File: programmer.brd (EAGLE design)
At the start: 41.1 x 23 mm, 20 parts, among them IC1 74ABT125DB, U1 ATMEGA8U2, X1 16MHz

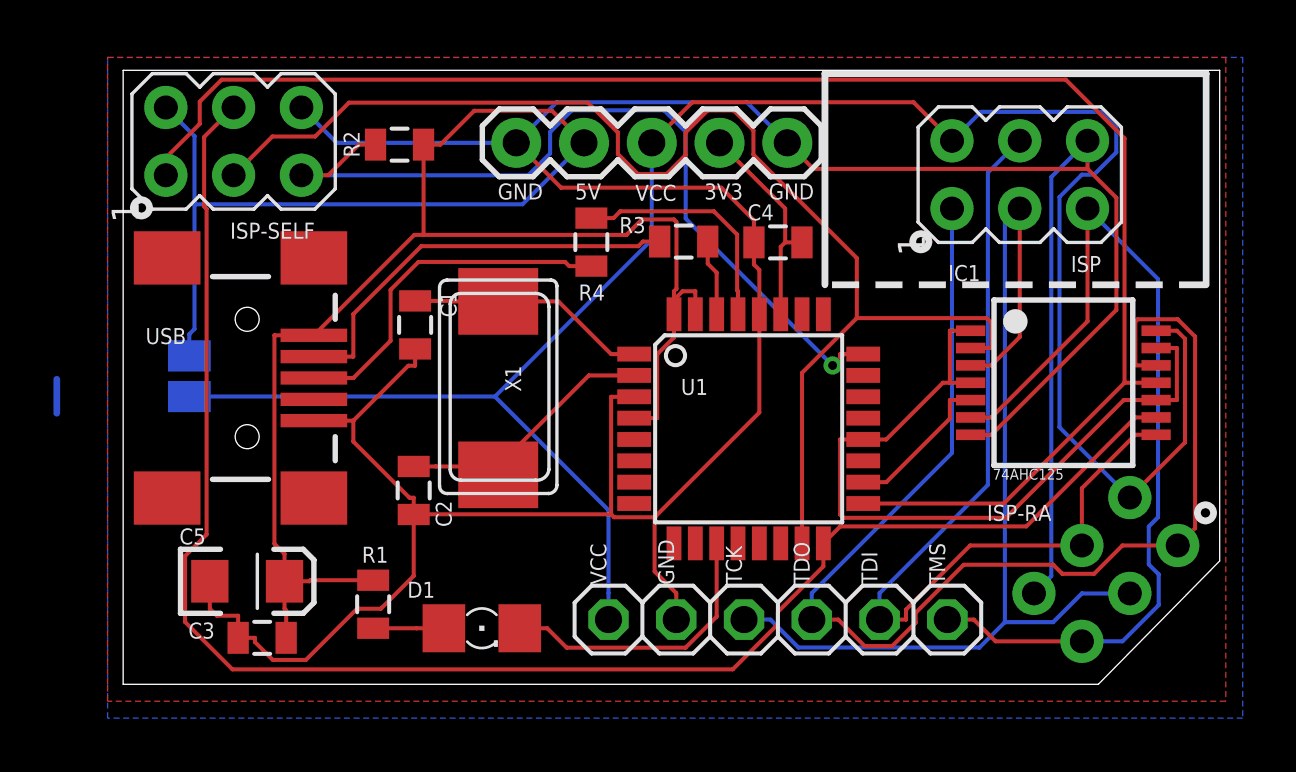
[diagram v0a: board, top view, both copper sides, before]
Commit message: v1.0s.  s for squished
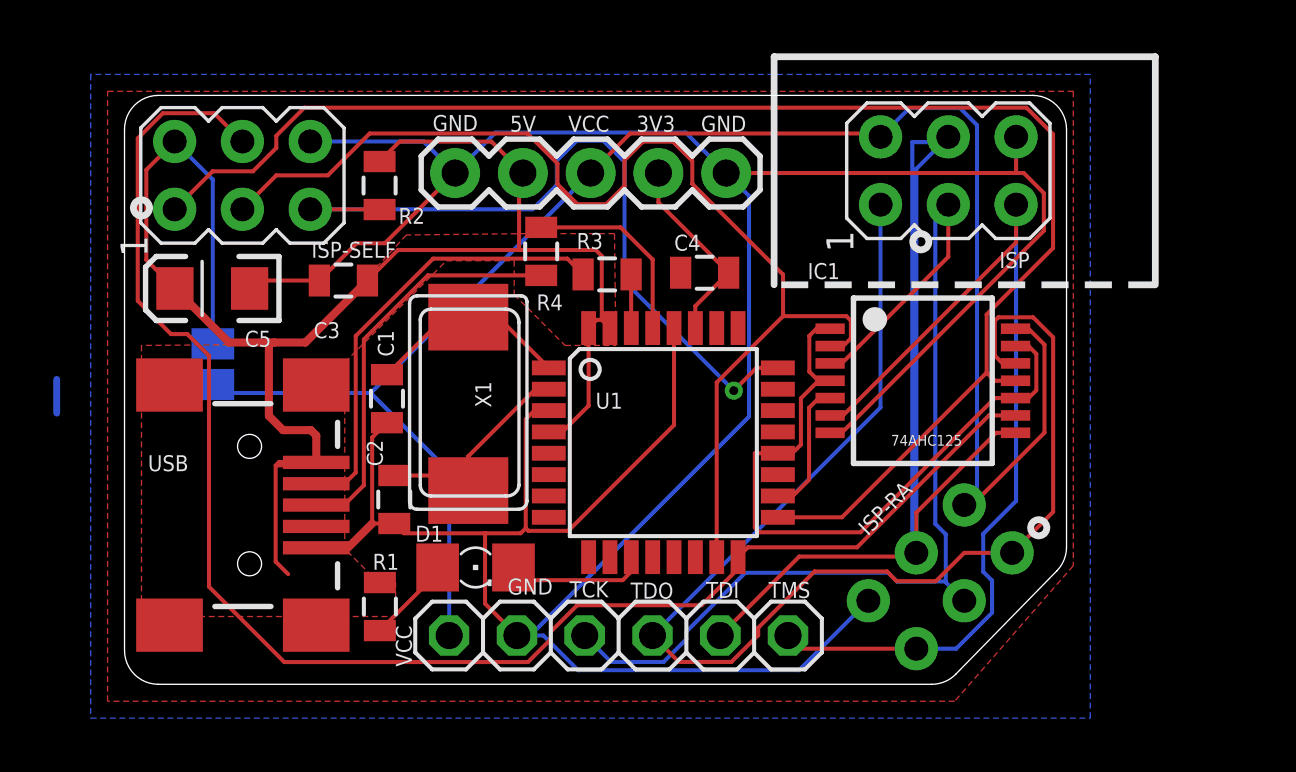
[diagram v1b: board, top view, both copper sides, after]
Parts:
- moved C3 13.7 mm to (8.20, 15.1)
- moved C5 11.1 mm to (3.29, 14.8), turned to 180 degrees
- moved ISP-RA 6.21 mm to (30.6, 4.03)
- moved JP2 6.00 mm to (18.5, 1.83)
- moved IC1 5.27 mm to (29.9, 11.4)
- moved USB 4.76 mm to (4.69, 6.72)
- moved U1 3.24 mm to (20.2, 9.06)
- moved R3 3.12 mm to (18.1, 15.4)
- moved C4 2.97 mm to (21.7, 15.4)
- moved C1 2.96 mm to (9.84, 10.7)
- moved ISP 2.68 mm to (30.9, 19.2)
- moved JP1 2.56 mm to (12.4, 19.2)
- moved D1 2.29 mm to (13.2, 4.38)
- moved R4 1.91 mm to (15.6, 16.2)
- moved R2 1.71 mm to (9.56, 18.7), turned to 270 degrees
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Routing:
- net 5V: track 78.0 -> 64.1 mm
- net MOSI: track 34.8 -> 48.4 mm
- net VCC: track 77.0 -> 67.8 mm
- net GND: track 128.6 -> 121.7 mm
- net SCK-UC: track 48.8 -> 42.9 mm
- net ACTIVITY: track 10.9 -> 5.29 mm
- net MISO-UC: track 61.2 -> 56.4 mm
- net RESET: track 31.9 -> 28.6 mm
- net MOSI-UC: track 61.9 -> 58.7 mm
- net BUFFER-OE: track 28.5 -> 25.6 mm
- net MISO: track 46.8 -> 49.4 mm
- net XTAL2: track 10.00 -> 8.12 mm
- net D+RAW: track 13.4 -> 15.2 mm
- net D+: track 8.93 -> 7.25 mm
- net XTAL1: track 9.04 -> 7.75 mm
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- added copper zone on layer 1, net 5V
- added copper zone on layer 16, net GND
- removed copper zone on layer 16, net VCC
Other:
- board size 41.1 x 23 mm -> 35.3 x 22.1 mm
